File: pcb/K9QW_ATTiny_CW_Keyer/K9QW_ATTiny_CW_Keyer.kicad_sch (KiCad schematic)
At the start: 30 parts, among them J1 Paddle Input, J2 Key Output, J3 Command, J4 Sidetone, J5 Barrel_Jack_MountingPin, J6 Paddle Input, J7 Key Output, J8 LED, J9 Power Input, Q1 MMBT2222A, Q2 MMBT3904, Q3 MMBT3904, SW1 Command, SW2 Power Switch, U1 ATtiny85-20P, U2 LD1117S33TR_SOT223

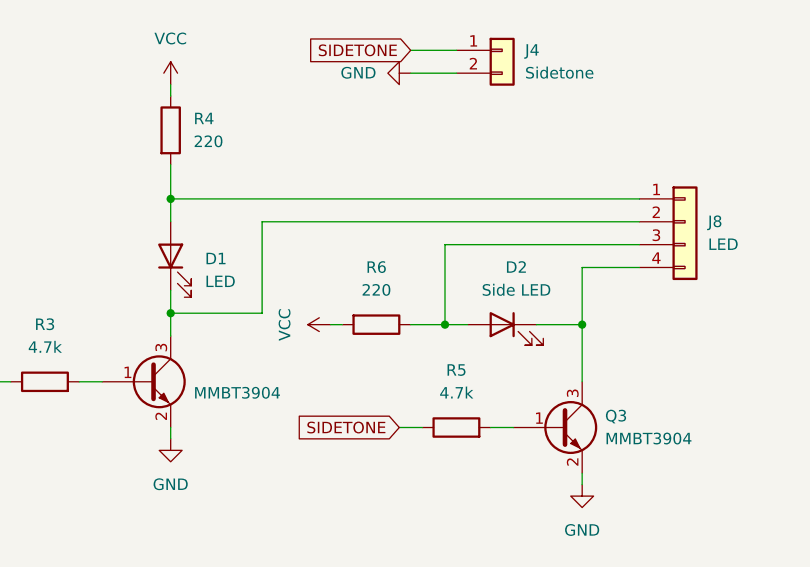
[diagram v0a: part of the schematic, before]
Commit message: Rough PCB Layout
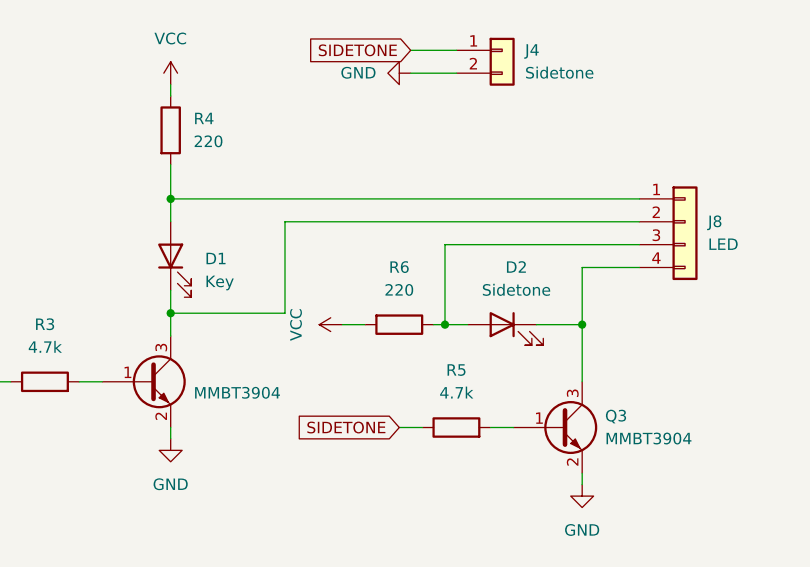
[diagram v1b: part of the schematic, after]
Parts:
- D1: value LED -> Key
- D2: value Side LED -> Sidetone
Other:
- moved on the sheet: R6
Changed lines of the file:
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@@
 	(wire
 		(pts
-			(xy 203.2 125.73) (xy 203.2 135.89)
+			(xy 205.74 125.73) (xy 205.74 135.89)
 		)
 		(stroke
@@
 	(wire
 		(pts
-			(xy 203.2 135.89) (xy 193.04 135.89)
+			(xy 205.74 135.89) (xy 193.04 135.89)
 		)
 		(stroke
@@
 	(wire
 		(pts
-			(xy 210.82 137.16) (xy 212.09 137.16)
+			(xy 212.09 137.16) (xy 214.63 137.16)
 		)
 		(stroke
@@
 	(wire
 		(pts
-			(xy 245.11 125.73) (xy 203.2 125.73)
+			(xy 245.11 125.73) (xy 205.74 125.73)
 		)
 		(stroke
@@
 	(wire
 		(pts
-			(xy 219.71 137.16) (xy 223.52 137.16)
+			(xy 222.25 137.16) (xy 223.52 137.16)
 		)
 		(stroke
@@
 			)
 		)
-		(property "Value" "LED"
+		(property "Value" "Key"
 			(at 196.85 132.3974 90)
 			(effects
@@
 	(symbol
 		(lib_id "power:VCC")
-		(at 210.82 137.16 90)
+		(at 212.09 137.16 90)
 		(unit 1)
 		(exclude_from_sim no)
@@
 		(dnp no)
 		(property "Reference" "#PWR020"
-			(at 214.63 137.16 0)
+			(at 215.9 137.16 0)
 			(effects
 				(font
@@
 		)
 		(property "Value" "VCC"
-			(at 205.74 137.16 0)
+			(at 207.01 137.16 0)
 			(effects
 				(font
@@
 		)
 		(property "Footprint" ""
-			(at 210.82 137.16 0)
+			(at 212.09 137.16 0)
 			(effects
 				(font
@@
 		)
 		(property "Datasheet" ""
-			(at 210.82 137.16 0)
+			(at 212.09 137.16 0)
 			(effects
 				(font
@@
 		)
 		(property "Description" "Power symbol creates a global label with name \"VCC\""
-			(at 210.82 137.16 0)
+			(at 212.09 137.16 0)
 			(effects
 				(font
@@
 			)
 		)
-		(property "Value" "Side LED"
+		(property "Value" "Sidetone"
 			(at 231.4575 133.35 0)
 			(effects
@@
 	(symbol
 		(lib_id "Device:R")
-		(at 215.9 137.16 270)
+		(at 218.44 137.16 270)
 		(unit 1)
 		(exclude_from_sim no)
@@
 		(fields_autoplaced yes)
 		(property "Reference" "R6"
-			(at 215.9 130.81 90)
+			(at 218.44 130.81 90)
 			(effects
 				(font
@@
 		)
 		(property "Value" "220"
-			(at 215.9 133.35 90)
+			(at 218.44 133.35 90)
 			(effects
 				(font
@@
 		)
 		(property "Footprint" "Resistor_SMD:R_0603_1608Metric_Pad0.98x0.95mm_HandSolder"
-			(at 215.9 135.382 90)
+			(at 218.44 135.382 90)
 			(effects
 				(font
@@
 		)
 		(property "Datasheet" "~"
-			(at 215.9 137.16 0)
+			(at 218.44 137.16 0)
 			(effects
 				(font
@@
 		)
 		(property "Description" "Resistor"
-			(at 215.9 137.16 0)
+			(at 218.44 137.16 0)
 			(effects
 				(font

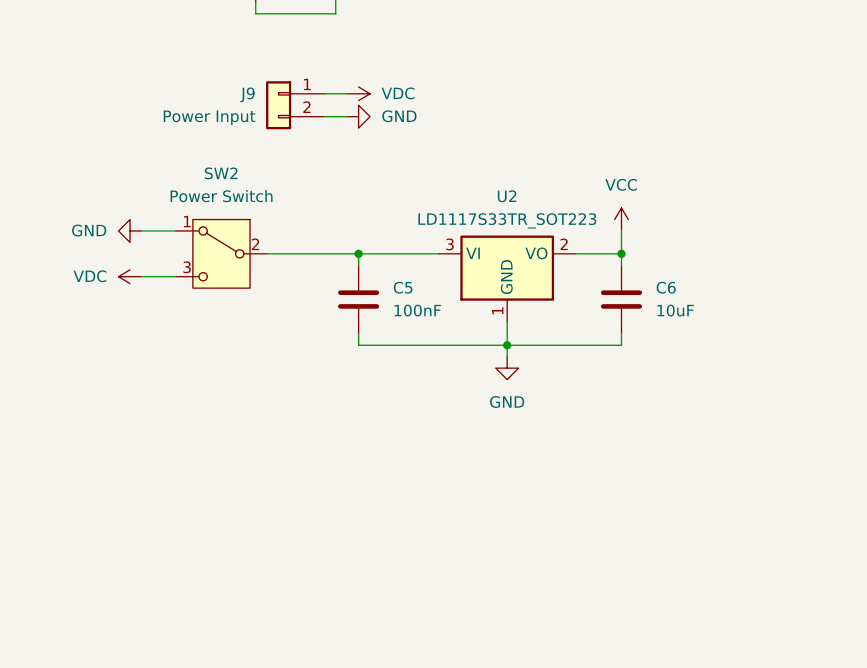
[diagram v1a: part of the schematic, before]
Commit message: Layout cleanup
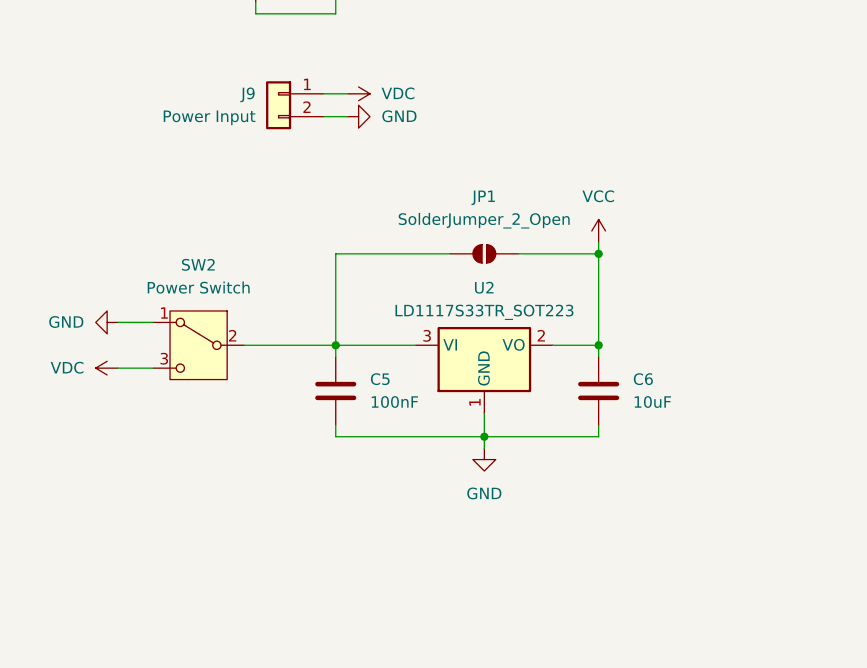
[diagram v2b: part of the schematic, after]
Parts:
- added JP1: SolderJumper_2_Open, Jumper:SolderJumper-2_P1.3mm_Open_RoundedPad1.0x1.5mm, symbol Jumper:SolderJumper_2_Open
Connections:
- net VCC: now also JP1.2 (B)
- net at C5.1, SW2.2 (B), U2.3 (VI): now also JP1.1 (A)
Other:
- moved on the sheet: C5, C6, SW2, U2
